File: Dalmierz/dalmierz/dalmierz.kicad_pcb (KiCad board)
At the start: 2 copper layers, 54 x 87 mm, 52 parts, among them J1 USB_B_Micro, J2 B4B-ZR_LF__SN_TF LUNA, J3 B4B-ZR_LF__SN_LCD I2C, J7 B4B-ZR_LF__SN_URM13, SW1 1-1825910-4, SW2 1-1825910-4, SW3 1-1825910-4, SW4 1-1825910-4, SW5 1-1825910-4, SW6 1-1825910-4, SW7 1-1825910-4, U1 RP2040, U2 RT6150B-33GQW, U4 W25Q32JVSS, U5 LC709203FQH-04TWG, U6 LM2775DSG, Y1 CSTNE12M0GH5L000R0

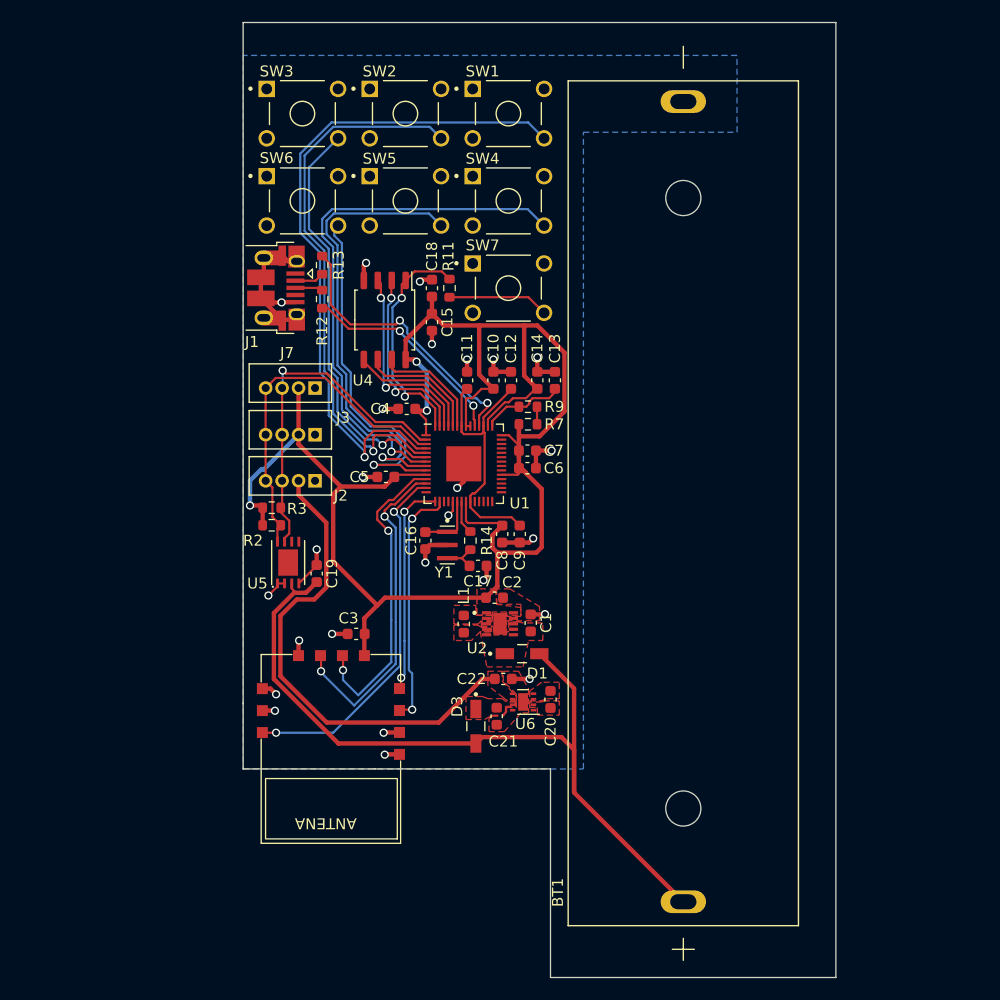
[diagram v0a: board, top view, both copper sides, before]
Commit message: MAIN: README dalmierz
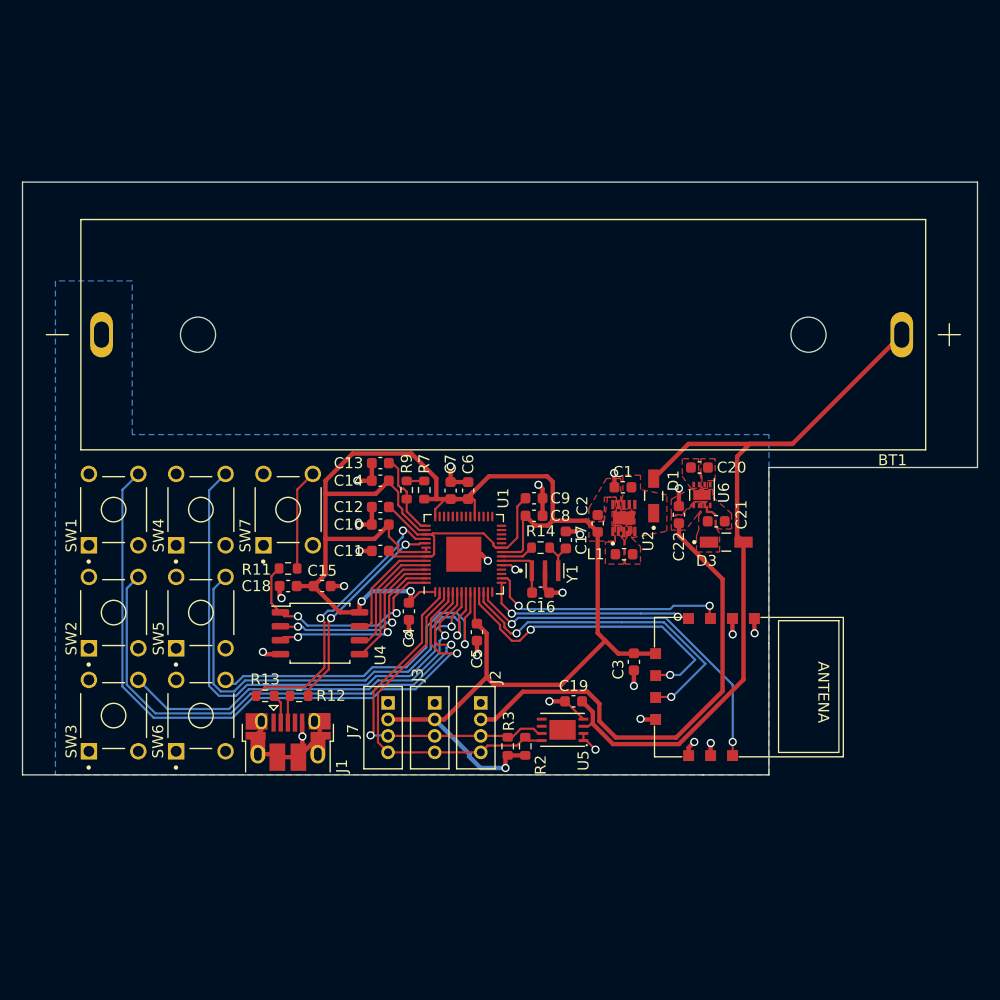
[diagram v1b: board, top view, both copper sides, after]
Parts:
- moved SW3 57.5 mm to (112.2, 124.1), turned to 90 degrees
- moved SW2 52.7 mm to (112.2, 114.8), turned to 90 degrees
- moved SW1 50.9 mm to (112.2, 105.4), turned to 90 degrees
- moved SW6 47.8 mm to (120.2, 124.1), turned to 90 degrees
- moved B1 43.9 mm to (175.3, 120.5), turned to 90 degrees
- moved SW5 41.9 mm to (120.2, 114.8), turned to 90 degrees
- moved J1 41.4 mm to (128.1, 126.5), turned to 0 degrees
- moved SW4 39.7 mm to (120.2, 105.4), turned to 90 degrees
- moved R13 39.6 mm to (126.0, 122.3), turned to 180 degrees
- moved R12 36.2 mm to (129.1, 122.3), turned to 0 degrees
- moved J7 32.5 mm to (136.8, 125.2), turned to 90 degrees
- moved R2 30.6 mm to (149.7, 126.9), turned to -90 degrees
- moved R3 30.6 mm to (148.1, 126.9), turned to 90 degrees
- moved C18 30.1 mm to (128.1, 112.3), turned to 180 degrees
- moved J3 30.0 mm to (141.0, 125.2), turned to 90 degrees
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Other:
- board size 54 x 87 mm -> 87 x 54 mm
